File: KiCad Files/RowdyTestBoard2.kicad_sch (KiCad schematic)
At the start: 0 parts

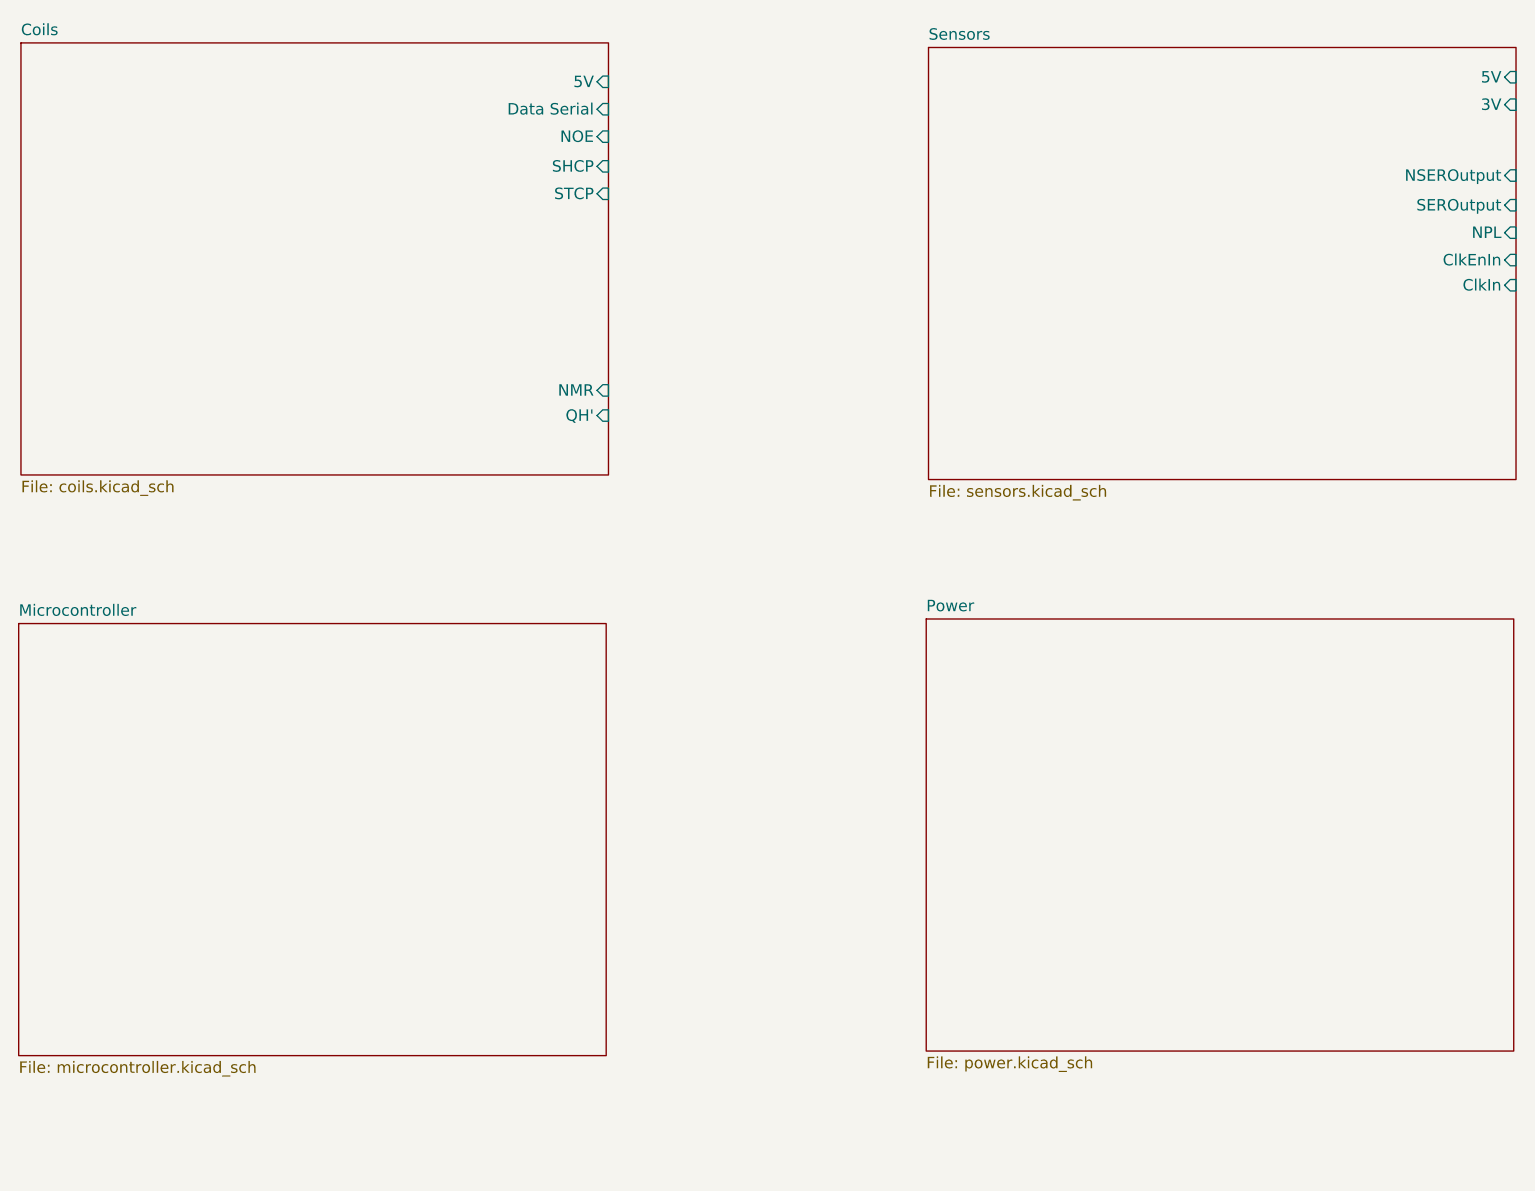
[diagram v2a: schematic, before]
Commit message: Pcb2
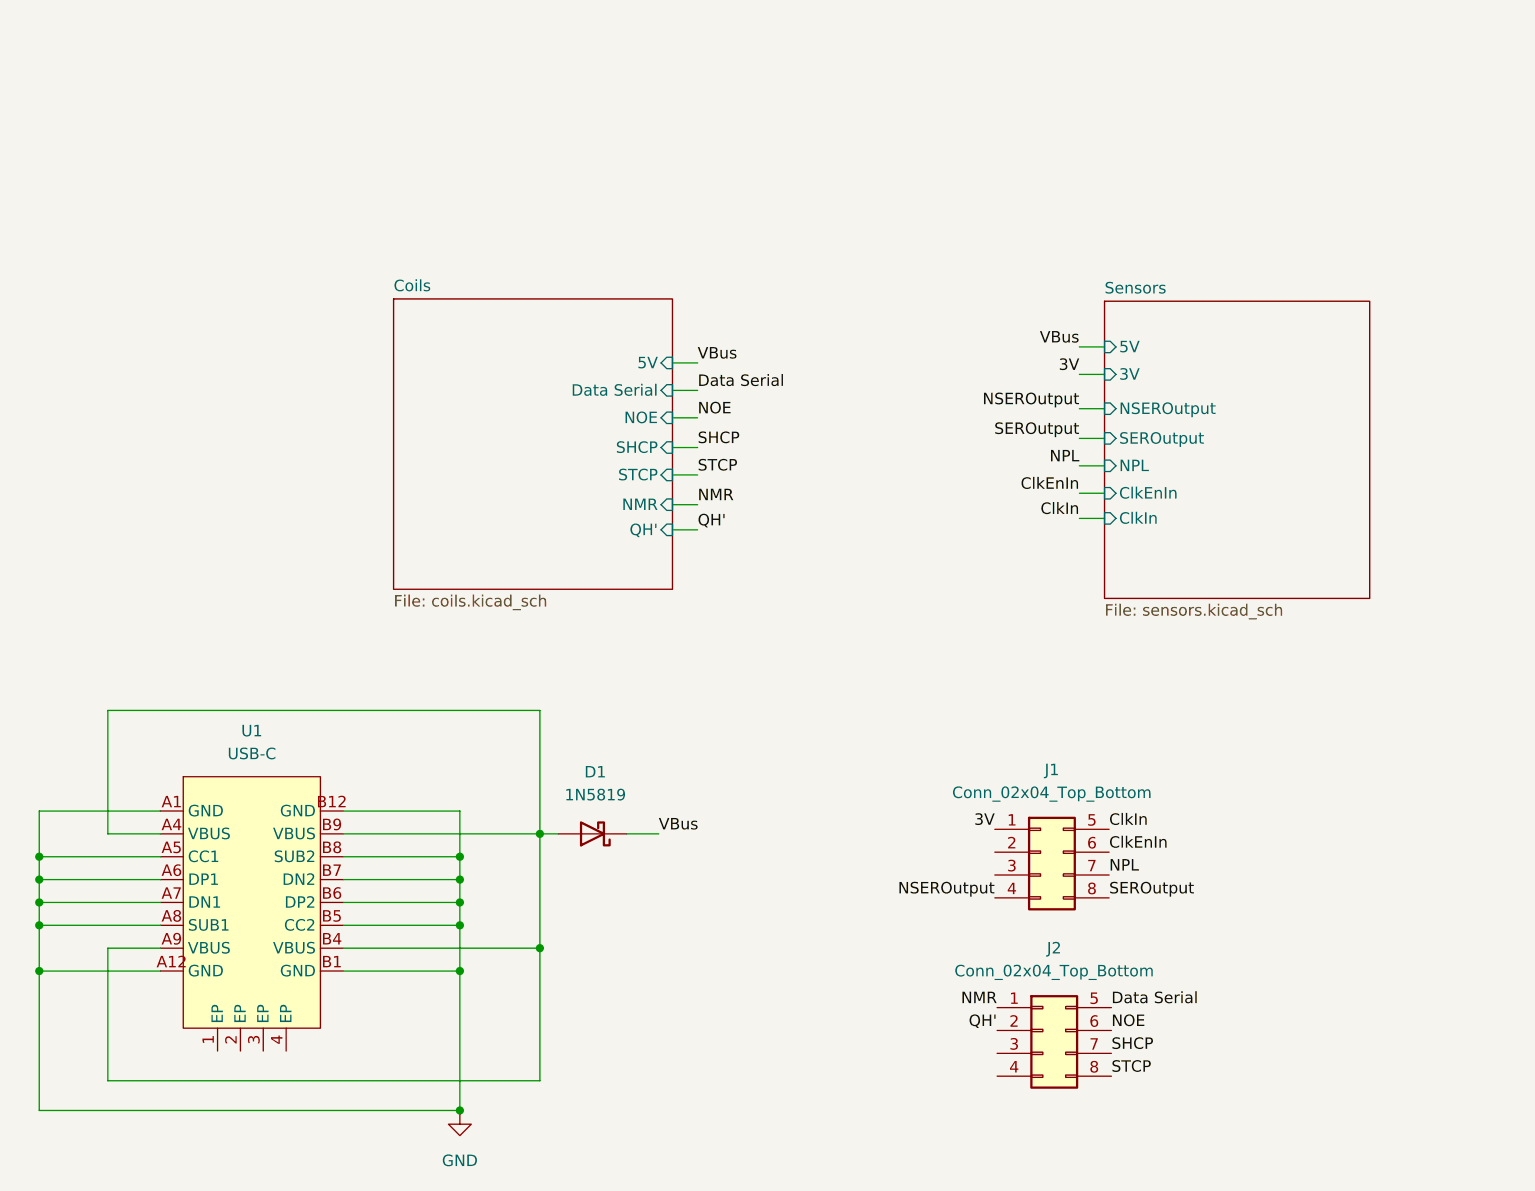
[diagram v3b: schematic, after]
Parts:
- added D1: 1N5819, Diode_THT:D_DO-41_SOD81_P10.16mm_Horizontal, symbol Diode:1N5819
- added J1, J2: Conn_02x04_Top_Bottom, Connector_PinHeader_2.54mm:PinHeader_2x04_P2.54mm_Vertical_SMD, symbol Connector_Generic:Conn_02x04_Top_Bottom
- added U1: USB-C, USB_C:USB-C-SMD_KH-TYPE-C-16P, symbol usb-c:USB-C
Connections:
- new net: D1.2 (A), U1.A4 (VBUS), U1.A9 (VBUS), U1.B4 (VBUS), U1.B9 (VBUS)
- new net 3V: J1.1 (Pin_1)
- new net ClkEnIn: J1.6 (Pin_6)
- new net ClkIn: J1.5 (Pin_5)
- new net Data Serial: J2.5 (Pin_5)
- new net GND: U1.A1 (GND), U1.A12 (GND), U1.A5 (CC1), U1.A6 (DP1), U1.A7 (DN1), U1.A8 (SUB1), U1.B1 (GND), U1.B12 (GND), U1.B5 (CC2), U1.B6 (DP2), U1.B7 (DN2), U1.B8 (SUB2)
- new net NMR: J2.1 (Pin_1)
- new net NOE: J2.6 (Pin_6)
- new net NPL: J1.7 (Pin_7)
- new net NSEROutput: J1.4 (Pin_4)
- new net QH': J2.2 (Pin_2)
- new net SEROutput: J1.8 (Pin_8)
- new net SHCP: J2.7 (Pin_7)
- new net STCP: J2.8 (Pin_8)
- new net VBus: D1.1 (K)
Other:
- removed sheet Microcontroller
- removed sheet Power

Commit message: diode
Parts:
- D1: footprint Diode_THT:D_DO-41_SOD81_P10.16mm_Horizontal -> Diode_SMD:D_SOD-323F; JLC Part Number (none) -> C2128
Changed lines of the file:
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@@
     (property "Reference" "D1" (id 0) (at 102.4255 115.824 0))
     (property "Value" "1N5819" (id 1) (at 102.4255 118.364 0))
-    (property "Footprint" "Diode_THT:D_DO-41_SOD81_P10.16mm_Horizontal" (id 2) (at 102.108 118.237 0)
+    (property "Footprint" "Diode_SMD:D_SOD-323F" (id 2) (at 102.108 118.237 0)
       (effects (font (size 1.27 1.27)) hide)
     )
     (property "Datasheet" "http://www.vishay.com/docs/88525/1n5817.pdf" (id 3) (at 102.108 122.682 0)
+      (effects (font (size 1.27 1.27)) hide)
+    )
+    (property "JLC Part Number" "C2128" (id 4) (at 102.108 122.682 0)
       (effects (font (size 1.27 1.27)) hide)
     )
@@
     )
     (path "/06df2c7b-9992-4fe2-8804-c49a5197fa1a"
-      (reference "D1") (unit 1) (value "1N5819") (footprint "Diode_THT:D_DO-41_SOD81_P10.16mm_Horizontal")
+      (reference "D1") (unit 1) (value "1N5819") (footprint "Diode_SMD:D_SOD-323F")
     )
     (path "/a6b1e09a-8af3-4cc4-9df1-f67a0e8f20fc/ff45e544-680d-4099-bd07-451c5137b60b"
-      (reference "IC1") (unit 1) (value "AH1902-Z-7") (footprint "AH1902Z7")
+      (reference "IC1") (unit 1) (value "AH1902-Z-7") (footprint "HallSensor:AH1902Z7")
     )
     (path "/a6b1e09a-8af3-4cc4-9df1-f67a0e8f20fc/266b7e6f-426b-43f7-b46d-50ac4ff256b9"
-      (reference "IC2") (unit 1) (value "AH1902-Z-7") (footprint "AH1902Z7")
+      (reference "IC2") (unit 1) (value "AH1902-Z-7") (footprint "HallSensor:AH1902Z7")
     )
     (path "/a6b1e09a-8af3-4cc4-9df1-f67a0e8f20fc/94b7b858-992d-497a-bd6b-051f4dea2255"
-      (reference "IC3") (unit 1) (value "AH1902-Z-7") (footprint "AH1902Z7")
+      (reference "IC3") (unit 1) (value "AH1902-Z-7") (footprint "HallSensor:AH1902Z7")
     )
     (path "/a6b1e09a-8af3-4cc4-9df1-f67a0e8f20fc/7b3f904b-56d8-43af-af24-37ea6851b116"
-      (reference "IC4") (unit 1) (value "AH1902-Z-7") (footprint "AH1902Z7")
+      (reference "IC4") (unit 1) (value "AH1902-Z-7") (footprint "HallSensor:AH1902Z7")
     )
     (path "/4afba3fc-9c59-47b9-9f58-f71bedabd29c"
